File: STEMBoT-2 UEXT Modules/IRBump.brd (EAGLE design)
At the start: 21.6 x 31.4 mm, 23 parts, among them IC1 LMV324DR2G, IC2 LMV324DR2G, IC3 74HC165PW,118, Q1 MMBT3904LP-7, U1 SN74HC148D

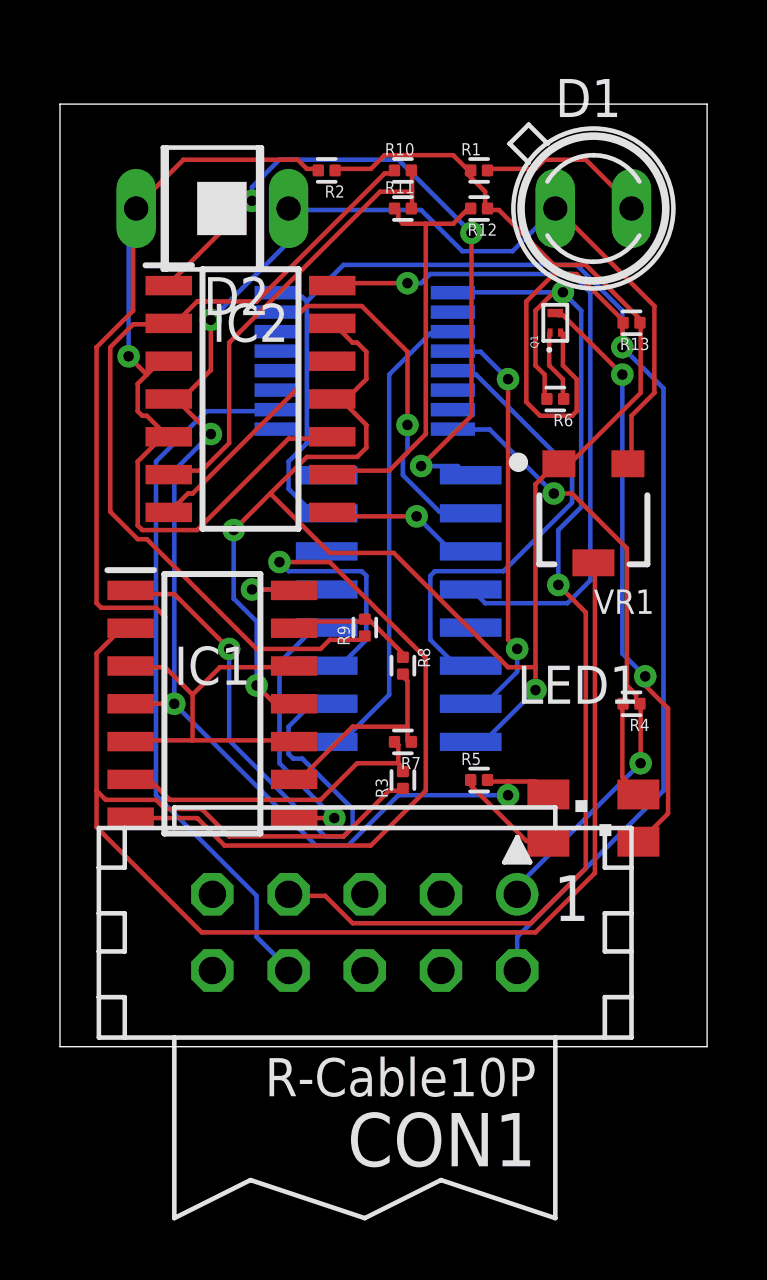
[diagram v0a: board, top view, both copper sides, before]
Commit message: Once again, updating ADC shematics and boards. Used autorouter.
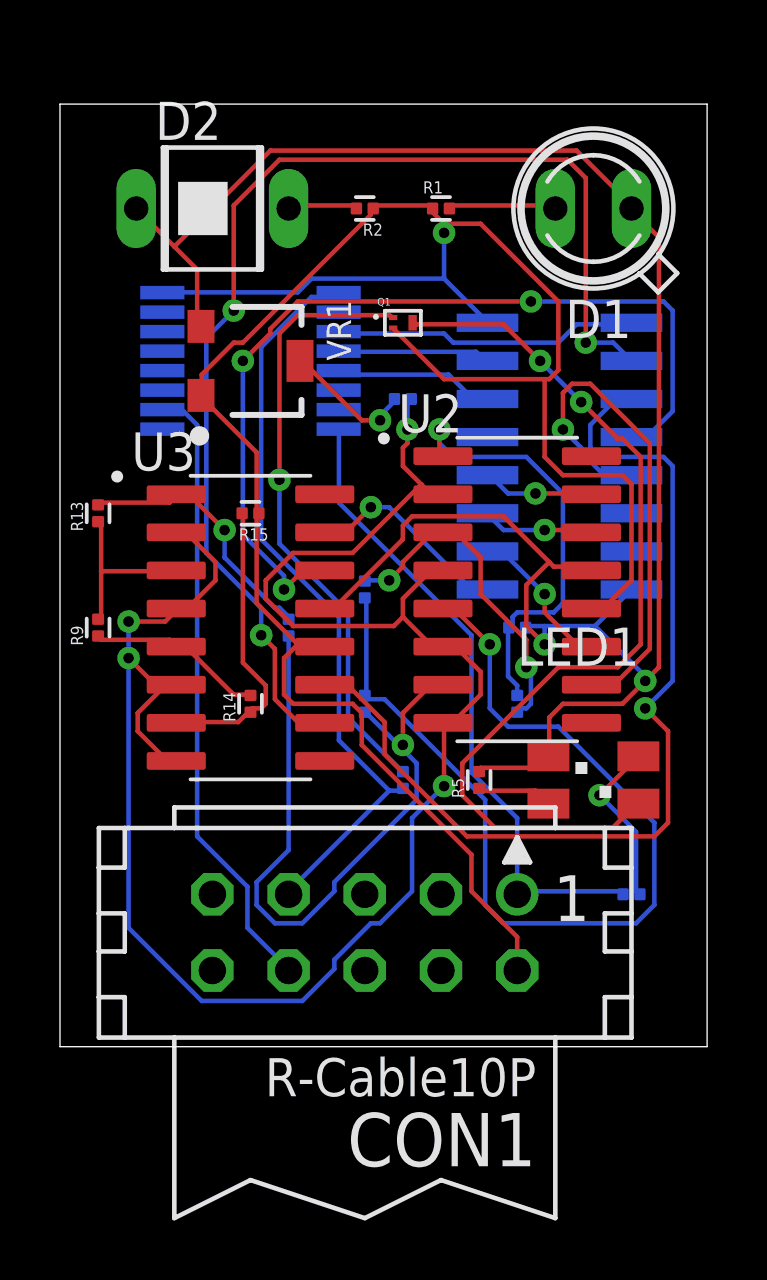
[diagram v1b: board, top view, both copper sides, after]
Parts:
- removed IC1, IC2: LMV324DR2G, LMV324DR2G:SOP126P600X175-14N
- added R14, R15: ERJ-1RHD3601C, Resistor:RESC0603X26N
- added U2, U3: MAX964ESET, MAX964ESET:SOIC127P600X175-16N
- moved R13 18.9 mm to (1.27, 17.8), turned to 90 degrees
- moved R10 18.2 mm to (15.2, 11.4), flipped to the bottom, turned to 270 degrees
- moved U1 17.3 mm to (19.1, 24.1), turned to 180 degrees
- moved R12 16.9 mm to (10.2, 11.4), flipped to the bottom, turned to 270 degrees
- moved R11 14.5 mm to (15.2, 14.0), flipped to the bottom
- moved R6 13.7 mm to (11.4, 8.89), flipped to the bottom, turned to 270 degrees
- moved R3 12.7 mm to (11.4, 21.6), flipped to the bottom, turned to 180 degrees
- moved VR1 12.5 mm to (6.35, 22.9), turned to 270 degrees
- moved R9 8.89 mm to (1.27, 14.0)
- moved R4 6.35 mm to (19.1, 5.08), flipped to the bottom
- moved R7 5.39 mm to (7.62, 14.0), flipped to the bottom, turned to 90 degrees
- moved Q1 5.08 mm to (11.4, 24.1), turned to 0 degrees
- moved IC3 3.81 mm to (6.35, 22.9)
- moved R8 2.84 mm to (10.2, 15.2), flipped to the bottom
- moved R1 1.80 mm to (12.7, 27.9)
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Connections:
- removed net N$21: IC1.11, IC2.11, IC2.13, R1.1, R12.1, R13.1, R2.1, U1.8, VR1.1
- removed net VCC: U1.16
- new net N$27: U1.12, U3.14
- new net N$32: U1.11, U3.11
- new net N$33: U1.10, U3.10
- net N$1: now also R3.2, U2.2, U2.4, U2.6, U2.8, U3.2, U3.4, U3.6, U3.8; no longer IC2.8, U1.3
- net N$11: now also R10.2, R8.1, U2.3; no longer IC2.1, U1.1
- net N$13: now also R12.1, R8.2, U2.5; no longer IC2.7, U1.2
- net N$14: no longer IC1.2
- net N$15: now also R12.2, R7.1, U2.7; no longer IC1.6, R3.2, R7.2
- net N$16: now also R13.2, R7.2, U3.1; no longer IC1.9, R7.1, R8.2
- net N$18: now also R13.1, U3.3; no longer IC1.13, R8.1
- net N$19: now also R14.2, U3.5; no longer IC2.2, R10.1
- net N$20: now also R14.1, R15.2, U3.7; no longer IC2.6, R10.2, R11.2
- net N$22: now also U1.3, U2.14; no longer IC1.14, U1.13
- net N$23: now also U1.2, U2.11; no longer IC1.8, U1.12
- net N$24: now also U1.13, U2.10; no longer IC1.7, U1.11
- net N$25: now also U1.1, U3.15; no longer IC1.1, U1.10
- net N$4: now also R1.1, R15.1, R2.1, U1.8, U2.12, U3.12, VR1.1; no longer R13.2, U1.15
- net N$5: now also U1.4, U2.15; no longer IC2.9, R11.1, R12.2
- net N$6: now also R11.1, U1.16, U2.13, U3.13; no longer IC1.4, IC2.4
- net N$7: no longer IC1.10, IC1.12, IC1.3, IC1.5, IC2.10, IC2.3, IC2.5
- net N$9: now also R10.1, R11.2, U2.1; no longer IC2.14, U1.4
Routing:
- net N$21: track 60.2 -> 0.00 mm, vias 3 -> 0
- net N$1: track 5.17 -> 64.6 mm, vias 1 -> 4
- net N$7: track 58.8 -> 2.40 mm, vias 1 -> 0
- net N$14: track 48.1 -> 4.39 mm, vias 0 -> 1
- net N$33: track 0.00 -> 39.6 mm, vias 0 -> 3
- net N$32: track 0.00 -> 32.5 mm, vias 0 -> 1
- net N$27: track 0.00 -> 30.3 mm, vias 0 -> 3
- net N$19: track 28.0 -> 5.90 mm
- net N$12: track 2.42 -> 20.4 mm, vias 0 -> 1
- net N$4: track 58.8 -> 76.3 mm
- net N$31: track 39.2 -> 25.3 mm, vias 2 -> 0
- net N$13: track 19.8 -> 32.5 mm
- net N$15: track 10.8 -> 23.5 mm, vias 0 -> 1
- net N$11: track 23.4 -> 11.2 mm, vias 3 -> 2
- net N$25: track 18.7 -> 6.94 mm
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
